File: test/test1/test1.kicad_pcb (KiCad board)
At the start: 2 copper layers, 53.3 x 52.8 mm, 5 parts, among them U1 module_mpu6050

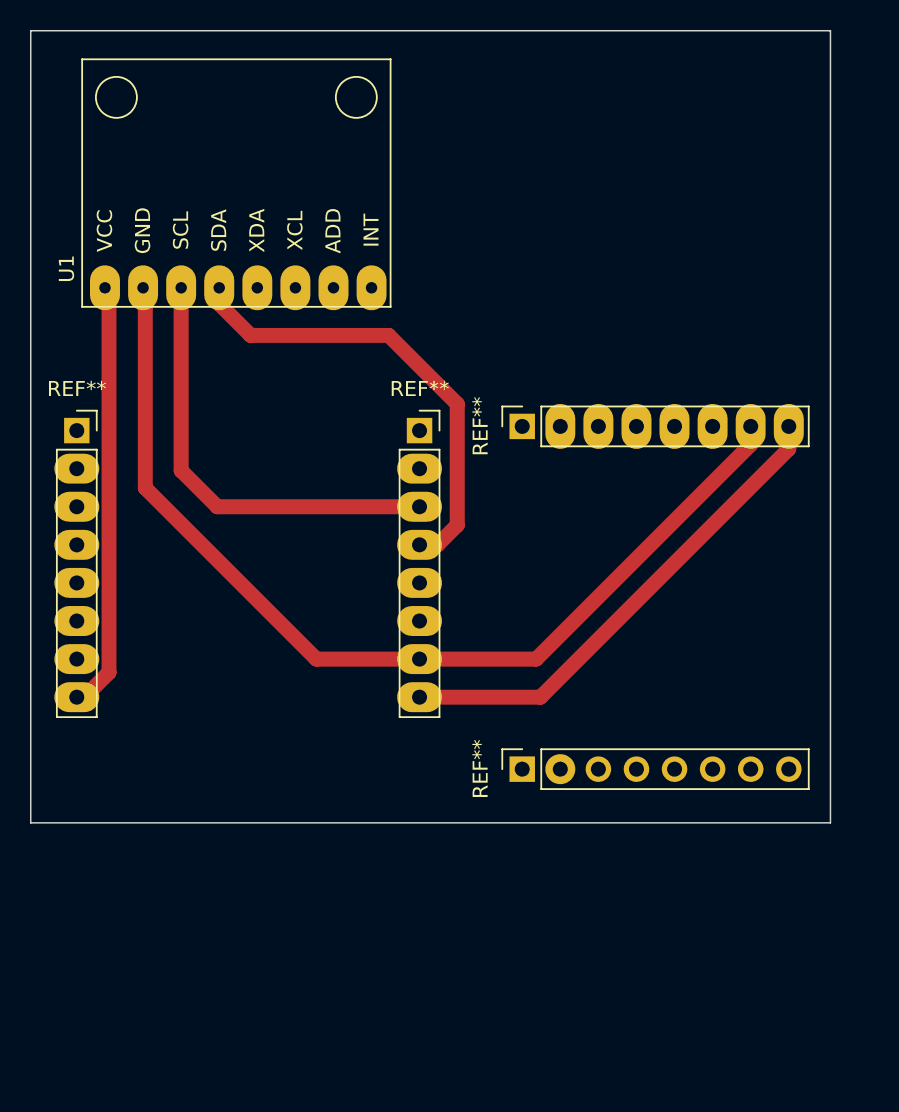
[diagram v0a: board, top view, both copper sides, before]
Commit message: tété
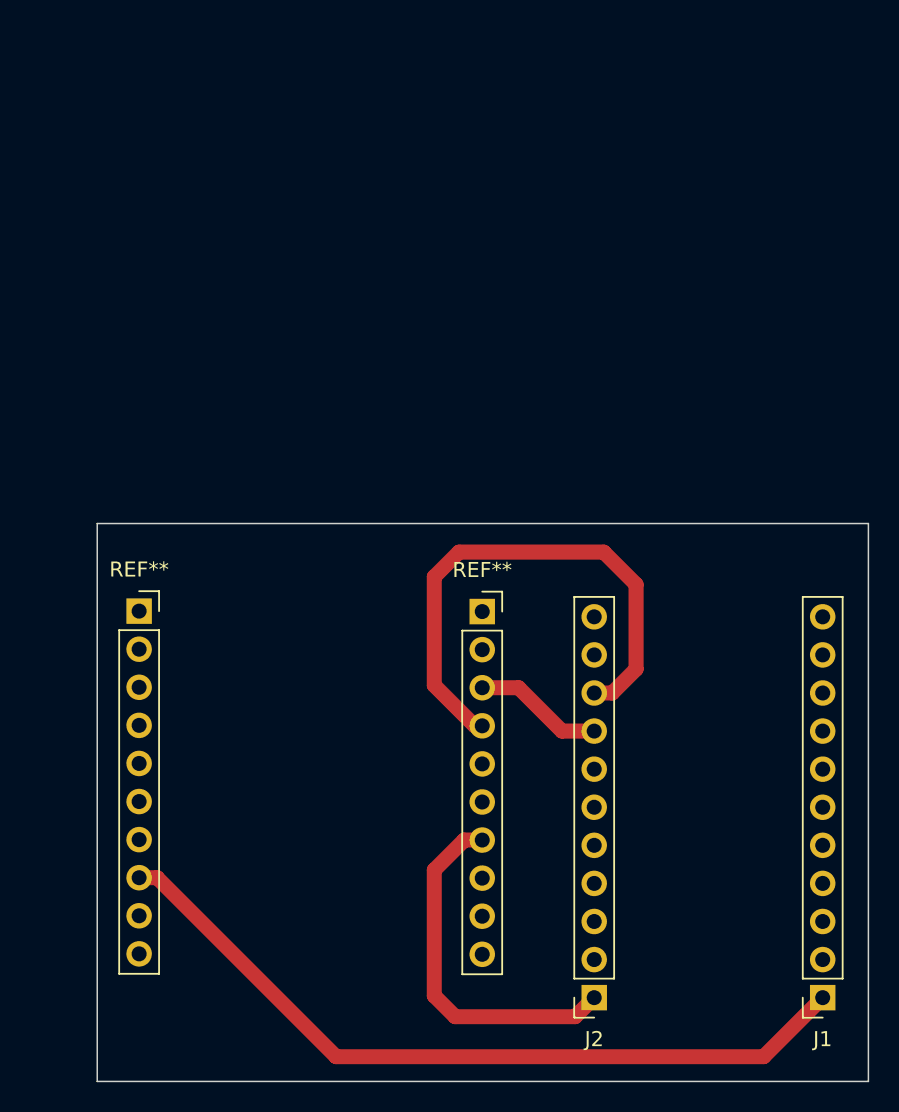
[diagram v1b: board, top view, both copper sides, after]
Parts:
- removed the REF** at (144.9, 71.8)
- removed the REF** at (144.9, 94.6)
- removed the REF** at (138.1, 72.0)
- removed the REF** at (115.2, 72.0)
- removed U1: module_mpu6050, usini_sensors:module_mpu6050
- added J1: Conn_01x12, Connector_PinSocket_2.54mm:PinSocket_1x11_P2.54mm_Vertical, F.Cu at (165.0, 109.9)
- added J2: Conn_01x12, Connector_PinSocket_2.54mm:PinSocket_1x11_P2.54mm_Vertical, F.Cu at (149.7, 109.9)
- added REF**: PinSocket_1x10_P2.54mm_Vertical, Connector_PinSocket_2.54mm:PinSocket_1x10_P2.54mm_Vertical, F.Cu at (142.3, 84.1)
- added REF**: PinSocket_1x10_P2.54mm_Vertical, Connector_PinSocket_2.54mm:PinSocket_1x10_P2.54mm_Vertical, F.Cu at (119.4, 84.1)
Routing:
- net GND: track 65.7 -> 24.7 mm
- net SDA: track 0.00 -> 35.7 mm
- net (no net): track 33.0 -> 0.00 mm
- net Net-(U1-Pad4): track 30.9 -> 0.00 mm
- net Net-(U1-Pad3): track 29.1 -> 0.00 mm
- net 3v3: track 28.6 -> 52.2 mm
- net SCL: track 0.00 -> 8.67 mm
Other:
- board size 53.3 x 52.8 mm -> 51.4 x 37.2 mm
